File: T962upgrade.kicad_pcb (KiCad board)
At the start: 2 copper layers, 82.9 x 51 mm, 91 parts, among them J1 Thermalcouple Screw Terminal, J2 2,54mm Pin Header, J3 GPIO Screw Terminal, J4 USB_B_Micro, J5 Fan In, J6 Fan Out, Q1 2N7002, SW1 Boot, SW2 Boot, U1 MAX31850KATB+, U2 CH340C, U3 LM1117-3.3, U4 LM1117-3.3, U5 MAX31850KATB+, U6 MAX31850KATB+, U7 MAX31850KATB+, U8 DS18S20

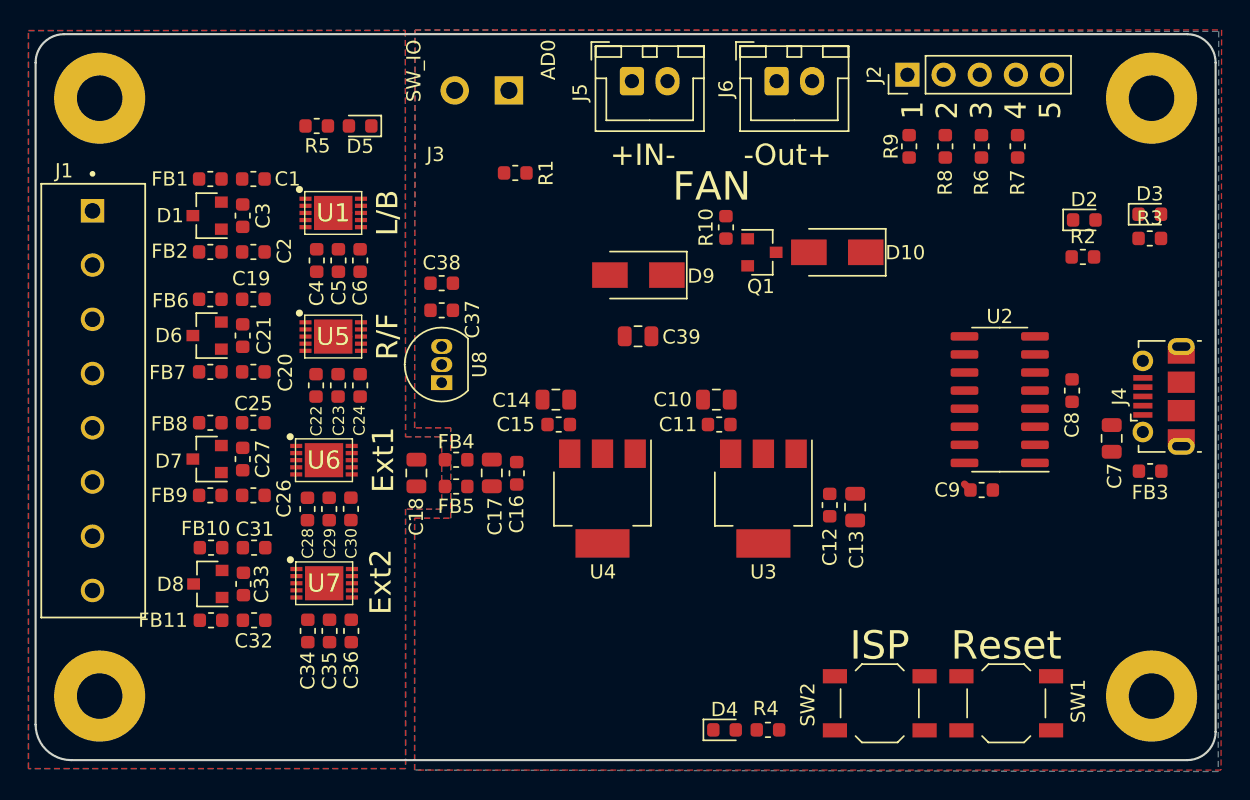
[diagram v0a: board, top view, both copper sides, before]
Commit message: Layout changes
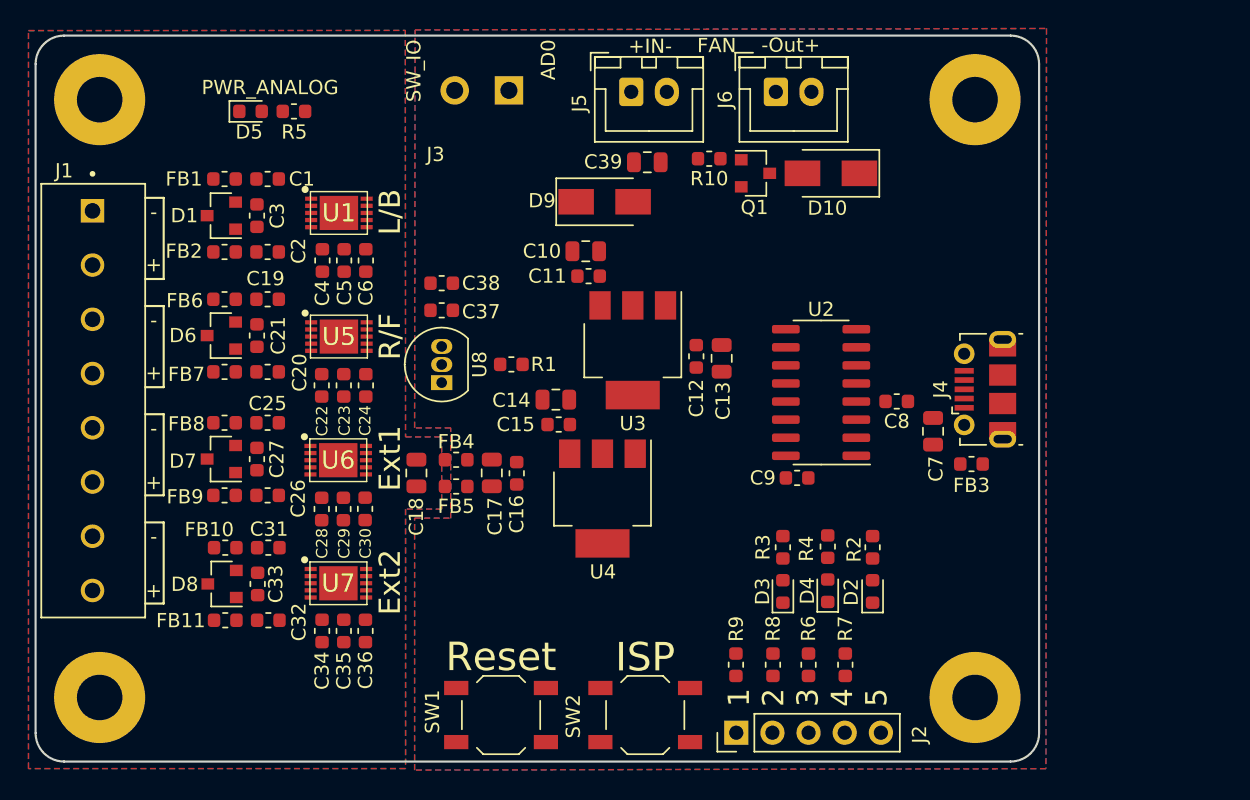
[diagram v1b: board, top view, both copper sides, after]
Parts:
- moved J2 47.8 mm to (153.7, 126.5)
- moved R9 38.4 mm to (153.7, 121.7), turned to 270 degrees
- moved R6 38.4 mm to (158.8, 121.7), turned to 270 degrees
- moved R8 38.4 mm to (156.3, 121.7), turned to 270 degrees
- moved R7 38.4 mm to (161.4, 121.7), turned to 270 degrees
- moved D3 37.0 mm to (157.0, 116.5), turned to 90 degrees
- moved SW1 35.5 mm to (137.2, 125.2)
- moved R3 33.7 mm to (157.0, 113.5), turned to 270 degrees
- moved D2 30.0 mm to (163.3, 116.5), turned to 90 degrees
- moved R2 25.2 mm to (163.3, 113.5), turned to 270 degrees
- moved SW2 16.5 mm to (147.3, 125.2)
- moved C12 14.0 mm to (150.9, 100.0)
- moved C13 14.0 mm to (152.7, 100.2)
- moved C11 13.9 mm to (143.3, 94.4)
- moved C10 13.9 mm to (143.2, 92.7)
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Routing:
- net VDD: track 0.80 -> 0.21 mm
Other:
- board size 82.9 x 51 mm -> 70.5 x 51 mm
- board text added: "+"
- board text added: "-"
- board text added: "PWR_ANALOG"
